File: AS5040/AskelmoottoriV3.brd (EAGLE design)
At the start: 50.1 x 48.6 mm, 15 parts, among them IC1 AS5040

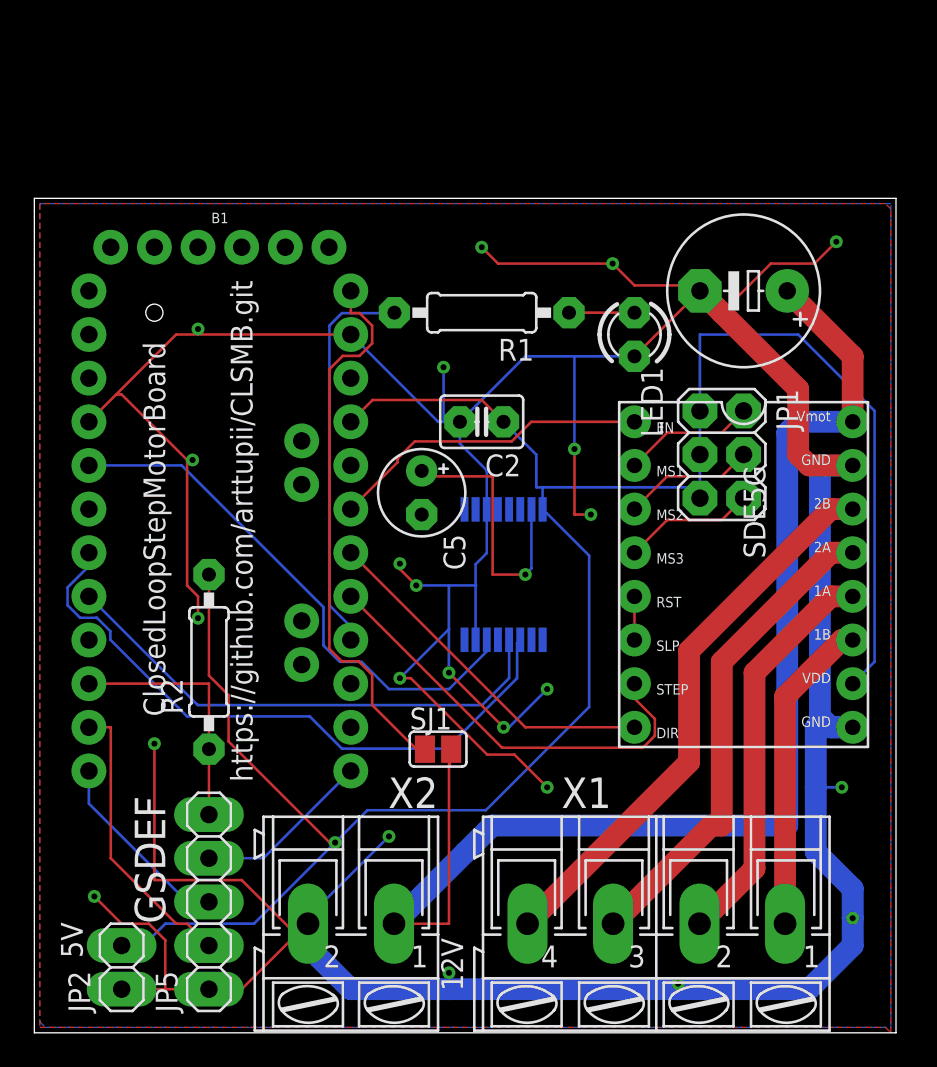
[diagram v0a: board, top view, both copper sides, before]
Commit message: Add crosshair
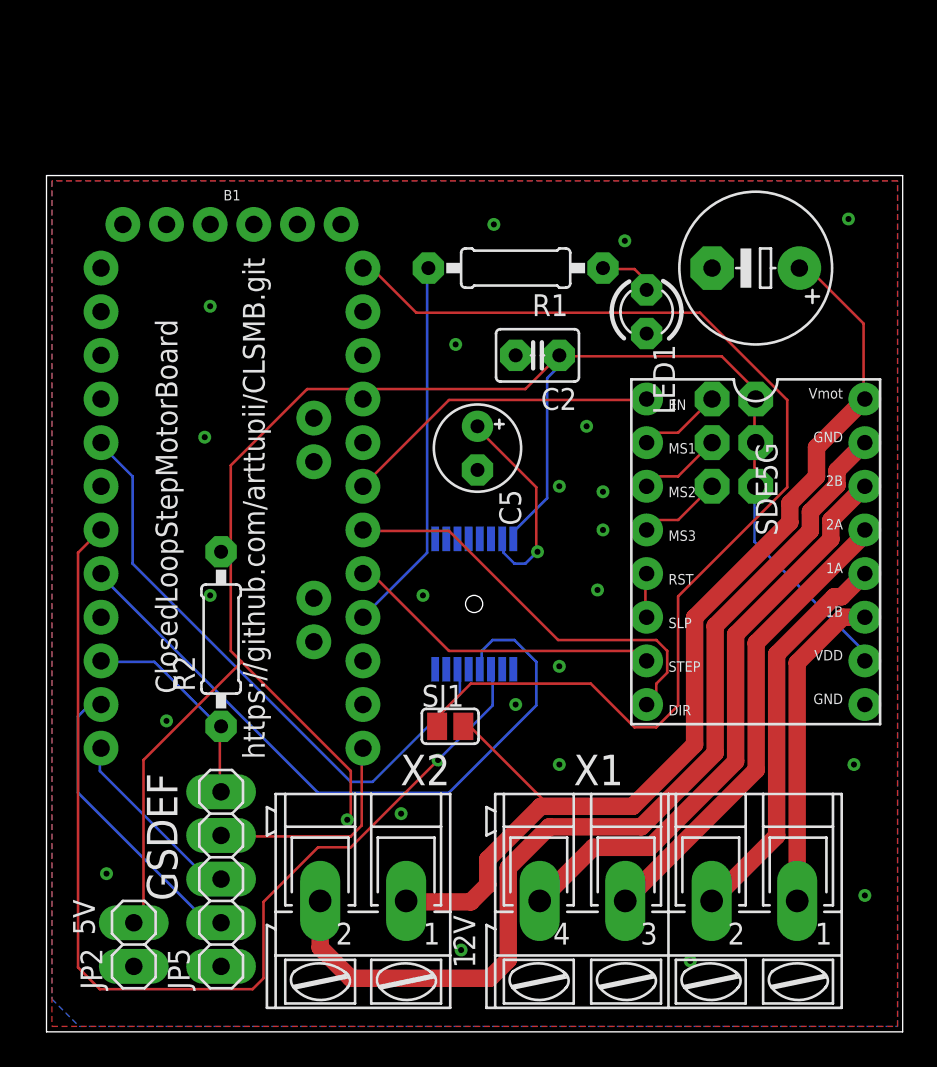
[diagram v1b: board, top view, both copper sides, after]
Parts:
- moved C2 5.05 mm to (28.6, 39.4)
- moved C5 4.16 mm to (25.2, 34.0)
- moved R1 3.26 mm to (27.4, 44.5)
- moved IC1 2.42 mm to (25.0, 25.0)
- moved R2 1.50 mm to (10.2, 22.9)
- moved LED1 1.50 mm to (35.0, 42.0)
- moved U$1 1.50 mm to (46.4, 35.6)
- moved X2 1.50 mm to (18.5, 7.68)
- moved JP2 1.50 mm to (5.15, 5.14)
- moved JP5 1.50 mm to (10.2, 8.95)
- moved B1 1.50 mm to (10.9, 31.8)
- moved SJ1 1.50 mm to (23.6, 17.8)
- moved X1 1.50 mm to (36.3, 7.68)
- moved C1 1.50 mm to (41.3, 44.5)
- moved JP1 0.99 mm to (40.1, 34.3), flipped to the bottom
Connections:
- net GND: now also IC1.10
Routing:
- net GND: track 275.5 -> 56.7 mm
- net N$14: track 32.3 -> 65.2 mm
- net N$5: track 37.5 -> 62.2 mm, vias 0 -> 1
- net +5V: track 127.7 -> 107.9 mm
- net +12V: track 76.1 -> 62.3 mm
- net N$6: track 30.0 -> 40.4 mm
- net N$8: track 25.2 -> 18.9 mm
- net N$17: track 31.5 -> 35.8 mm
- net N$15: track 15.8 -> 12.2 mm
- net N$9: track 20.7 -> 24.2 mm
- net N$12: track 7.67 -> 4.86 mm
- net N$16: track 7.67 -> 4.86 mm
- net N$13: track 7.67 -> 4.86 mm
- net EN: track 10.4 -> 13.0 mm
- net FEED_HOLD: track 14.6 -> 12.4 mm
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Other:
- board size 50.1 x 48.6 mm -> 49.8 x 49.8 mm
